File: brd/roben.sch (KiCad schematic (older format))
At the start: 82 parts, among them J1 POWER IN, J10 1+, J11 1-, J12 2-, J13 2+, J2 +V, J3 GND, J4 +V, J5 GND, J6 A, J7 B, J8 C, J9 D, U2 SN754410N, U3 Ardunano

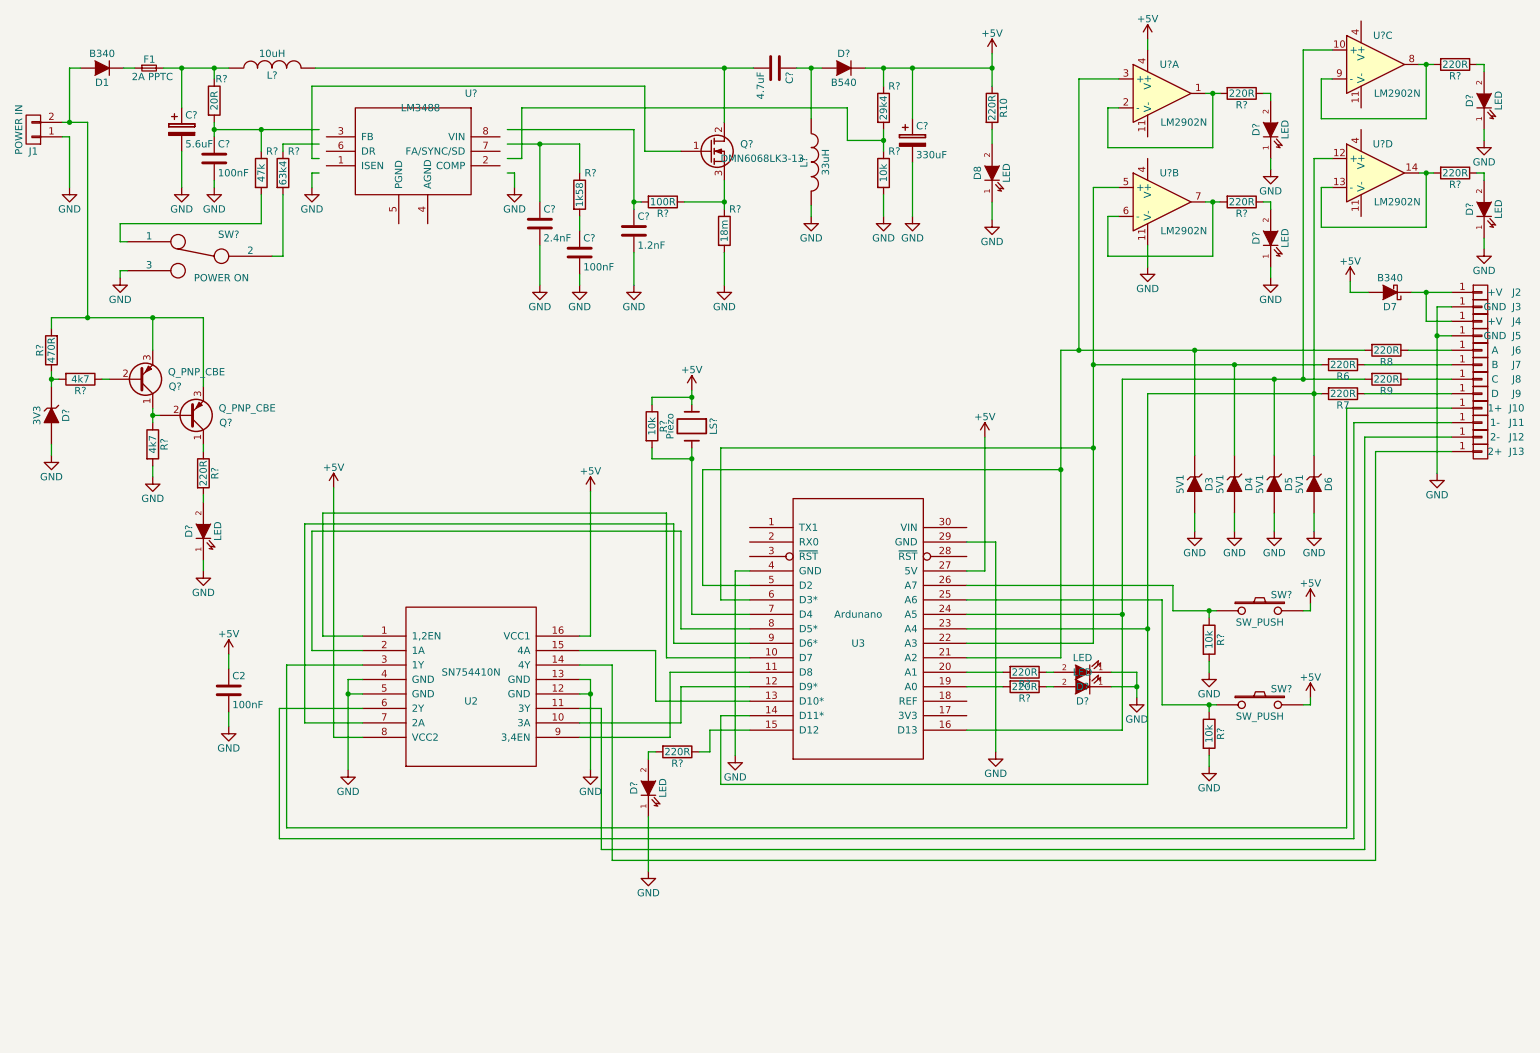
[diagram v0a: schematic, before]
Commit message: chg: optimizado esquemático y circuito
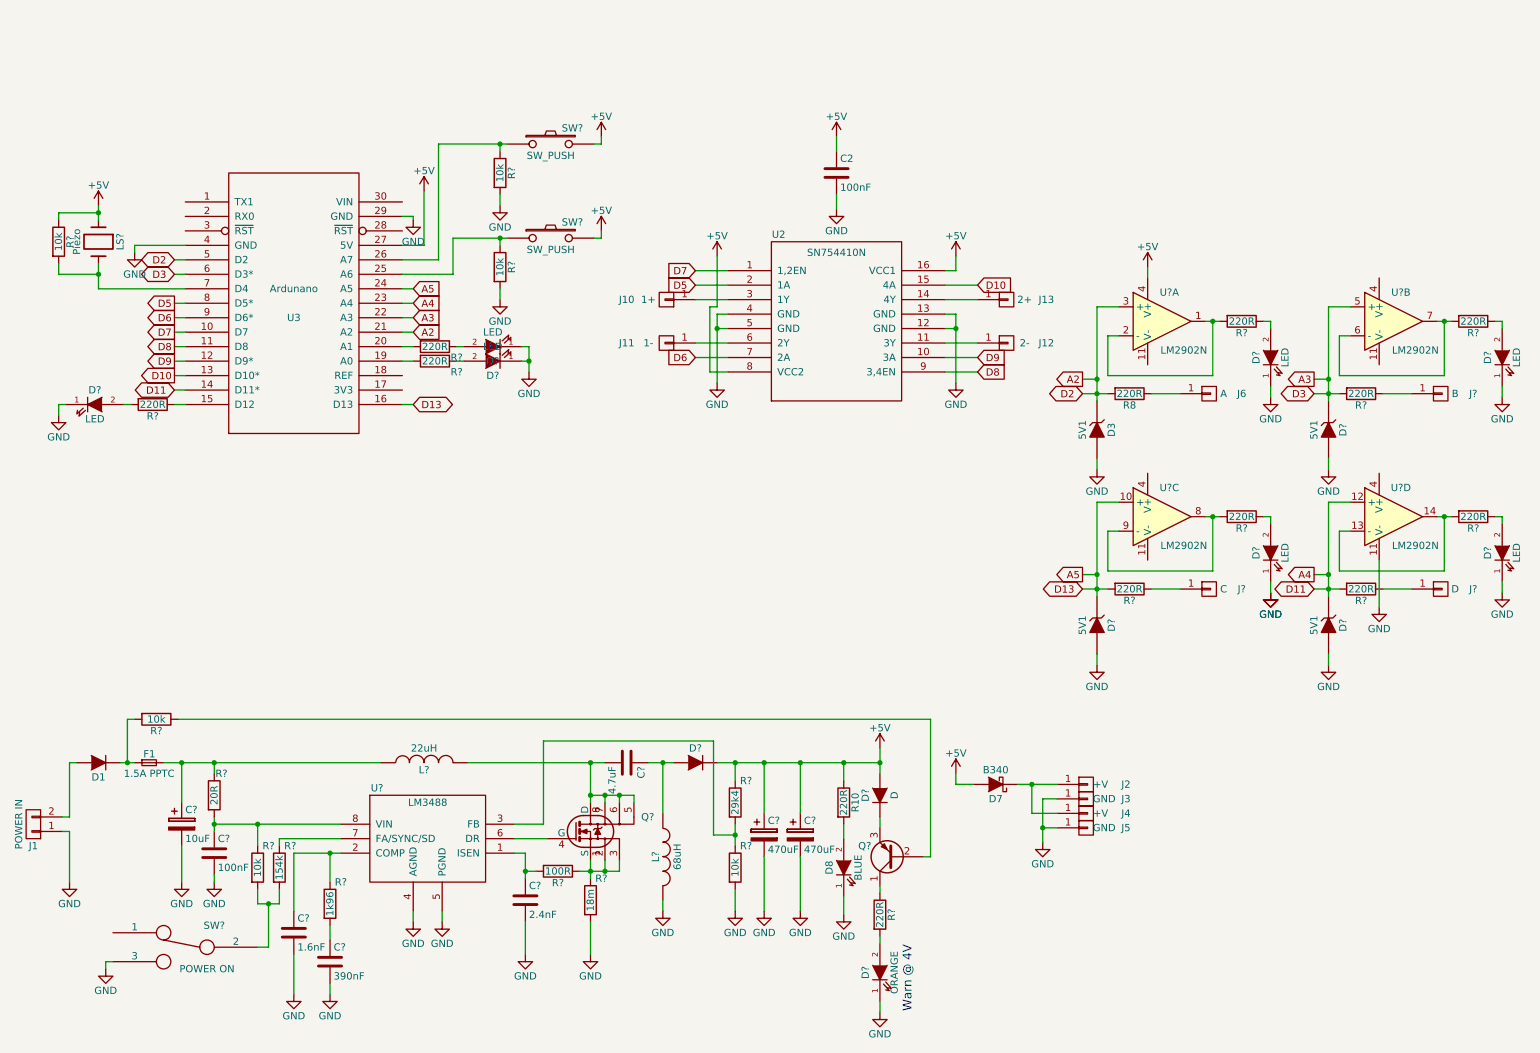
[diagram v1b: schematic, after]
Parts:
- removed D4, D5, D6: 5V1, Diodes_SMD:SOD-123, symbol ZENER
- removed D? (x3): LED, LEDs:LED-0805, symbol LED
- removed D?: 3V3, symbol ZENER
- removed J7: B, Wire_Pads:SolderWirePad_single_2-5mmDrill, symbol CONN_01X01
- removed J8: C, Wire_Pads:SolderWirePad_single_2-5mmDrill, symbol CONN_01X01
- removed J9: D, Wire_Pads:SolderWirePad_single_2-5mmDrill, symbol CONN_01X01
- removed Q?: DMN6068LK3-13, symbol Q_NMOS_GDS
- removed Q?: Q_PNP_CBE, symbol Q_PNP_CBE
- removed R6, R7, R9, R? (x3): 220R, Resistors_SMD:R_0805_HandSoldering, symbol R
- removed R?: 470R, symbol R
- removed R?: 4k7, symbol R
- removed U? (x3): LM2902N, symbol LM2902N
- added C?: 470uF, symbol CP
- added D?: D, symbol D
- added D? (x3): 5V1, Diodes_SMD:SOD-123, symbol ZENER
- added D? (x3): LED, LEDs:LED-0805, symbol LED
- added J?: B, Wire_Pads:SolderWirePad_single_2-5mmDrill, symbol CONN_01X01
- added J?: C, Wire_Pads:SolderWirePad_single_2-5mmDrill, symbol CONN_01X01
- added J?: D, Wire_Pads:SolderWirePad_single_2-5mmDrill, symbol CONN_01X01
- added Q?: BUK7Y98, LFPAK56, symbol IRF8721PBF-1
- added R? (x6): 220R, Resistors_SMD:R_0805_HandSoldering, symbol R
- added U? (x3): LM2902N, symbol LM2902N
- C?: Vendor (none) -> C0805C104K5RACTU
- C?: value 2.4nF -> 1.6nF; Vendor (none) -> GRM2165C1H162JA01D
- C?: value 100nF -> 390nF; Vendor (none) -> VJ0805Y394KXJTW1BC
- C?: Vendor (none) -> UMK316AB7475KL-T
- C?: value 1.2nF -> 2.4nF; Vendor (none) -> GRM2165C1H242JA01D
- C?: value 5.6uF -> 10uF; Vendor (none) -> VE-100M1HTR-0505
- C?: value 330uF -> 470uF; Vendor (none) -> UWT1A471MNL1GS
- D1: Vendor 621-B340-F -> B340-13-F
- D8: value LED -> BLUE; Vendor 720-LOR976-PS-1 -> LB Q39G-L2N2-35-1
- D?: value B540 -> SD2114S040S8R0; Vendor B540C-13-F -> SD2114S040S8R0
- D?: value LED -> ORANGE; Vendor 720-LOR976-PS-1 -> LO R976-PS-1
- F1: value 2A PPTC -> 1.5A PPTC; Vendor 530-0ZCF0200FF2C -> 0ZCF0150FF2C
- J1: Vendor 651-1985946 -> 1776493-2 / RAPC722X
- L?: value 33uH -> 68uH; Vendor (none) -> SDR1307-680KL
- L?: value 10uH -> 22uH; Vendor (none) -> SRR1210-220M
- Q?: value Q_PNP_CBE -> BC856; Vendor (none) -> BC856A-T
- R10: Vendor 71-CRCW0805-220-E3 -> ERJ-6GEYJ221V
- R?: Vendor (none) -> ERJ-6ENF20R0V
- R?: value 1k58 -> 1k96; Vendor (none) -> ERJ-6ENF1961V
- R?: Vendor (none) -> ERJ-6ENF2942V
- R?: Vendor (none) -> ERJ-6ENF1002V
- R?: value 63k4 -> 154k; Vendor (none) -> ERJ-6ENF1543V
- R?: Vendor (none) -> KRL1632E-M-R018-F-T5
- R?: Vendor (none) -> ERJ-6ENF1000V
- R?: value 47k -> 10k; Vendor (none) -> ERJ-6ENF1002V
- R?: Vendor (none) -> ERJ-6GEYJ221V
- R?: value 4k7 -> 10k; Vendor (none) -> ERJ-6ENF1002V
- SW?: Vendor (none) -> JS202011SCQN
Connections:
- net +5V: now also C?.1, D?.2 (A)
- net GND: now also U?.4 (AGND), U?.5 (PGND), C?.2, D?.1 (K), D?.1 (K), D?.1 (K), D?.2 (A), D?.2 (A), D?.2 (A), U?.11 (V-); no longer R?.2
- net D7: now reaches U2.1 (1,2EN), U3.10 (D7)
- net D9: now reaches U2.10 (3A), U3.12 (D9*)
- net D10: now reaches U2.15 (4A), U3.13 (D10*)
- net D5: now reaches U2.2 (1A), U3.8 (D5*)
- net D6: now reaches U2.7 (2A), U3.9 (D6*)
- net D8: now reaches U2.9 (3,4EN), U3.11 (D8)
- net at D1.2 (A), J1.2 (P2): no longer Q?.3 (E)
- net at D1.1 (K), F1.1: now also R?.2
- net A2: now reaches D3.1 (K), R8.2, U3.21 (A2), U3.5 (D2), U?.3 (+)
- net A5: now reaches U3.16 (D13), U3.24 (A5)
- net A5: now also D?.1 (K), R?.2, U?.10 (+)
- net A3: now reaches U3.22 (A3), U3.6 (D3*)
- net A3: now also D?.1 (K), R?.2, U?.5 (+)
- net A4: now reaches U3.14 (D11*), U3.23 (A4)
- net A4: now also D?.1 (K), R?.2, U?.12 (+)
- net at U?.1 (ISEN): now also C?.1, R?.2
- net at U?.2 (COMP): now also C?.1, R?.1
- net at U?.3 (FB): now also R?.1, R?.2
- net at U?.6 (DR): now also Q?.4 (G)
- net at U?.7 (FA/SYNC/SD): now also R?.1
- net at U?.8 (VIN): now also C?.1, R?.1, R?.2
- net at C?.2, L?.2: now also Q?.5, Q?.6, Q?.7, Q?.8 (D)
- net at R?.2, SW?.2: now also R?.2
- net at R?.1, R?.1: now also Q?.1 (S), Q?.2, Q?.3
- net at SW?.1: no longer R?.2
- new net: D?.1 (K), Q?.3 (E)
- new net: J?.1 (P1), R?.1 (x3)
- new net: R?.2, U?.6 (-), U?.7
- new net: D?.2 (A), R?.1 (x3)
- new net: R?.2, U?.8, U?.9 (-)
- new net: R?.2, U?.13 (-), U?.14
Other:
- note added: "Warn @ 4V"
- moved on the sheet: C2, C?, D1, D3, D7, D8, D?, F1, J1, J10, J11, J12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
